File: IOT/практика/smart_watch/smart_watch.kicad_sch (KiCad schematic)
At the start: 30 parts, among them J1 Conn_01x02_Pin, J2 USB_C_Receptacle_USB2.0_16P, SW3 SW_Push, U3 KXTJ3-1057, U4 MAX30102, U5 TPS61230DRC, U6 BQ24090DGQ, U7 ESP32-WROOM-32, U8 LC709203FQH-01TWG

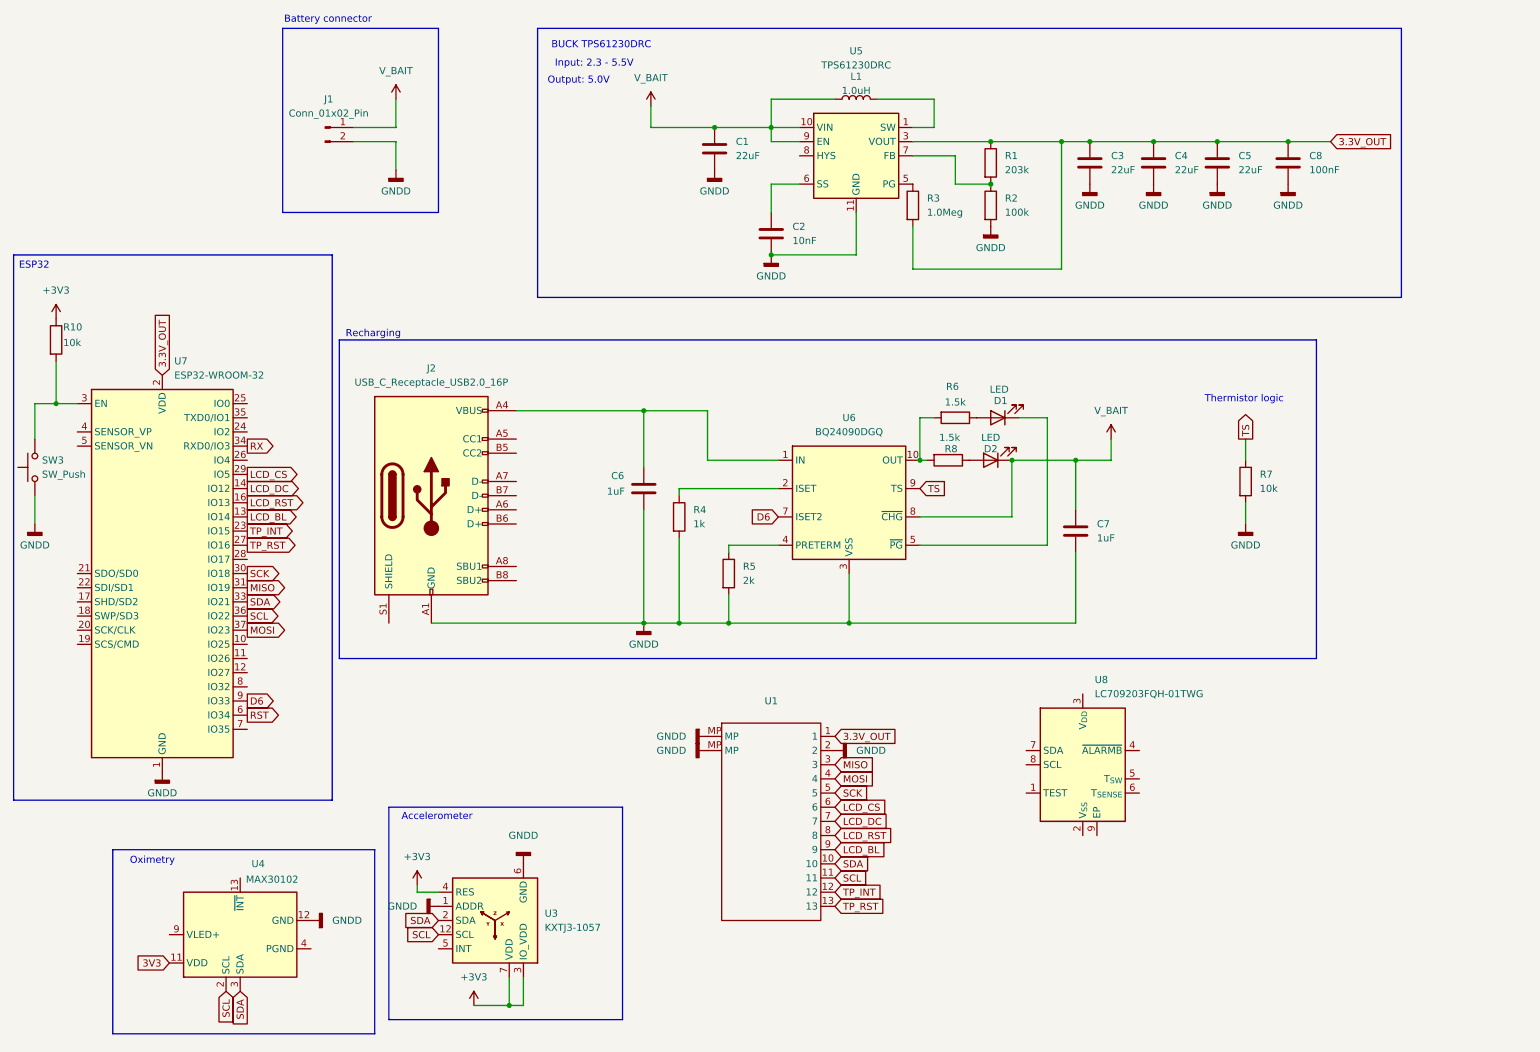
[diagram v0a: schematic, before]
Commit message: updating smart watch
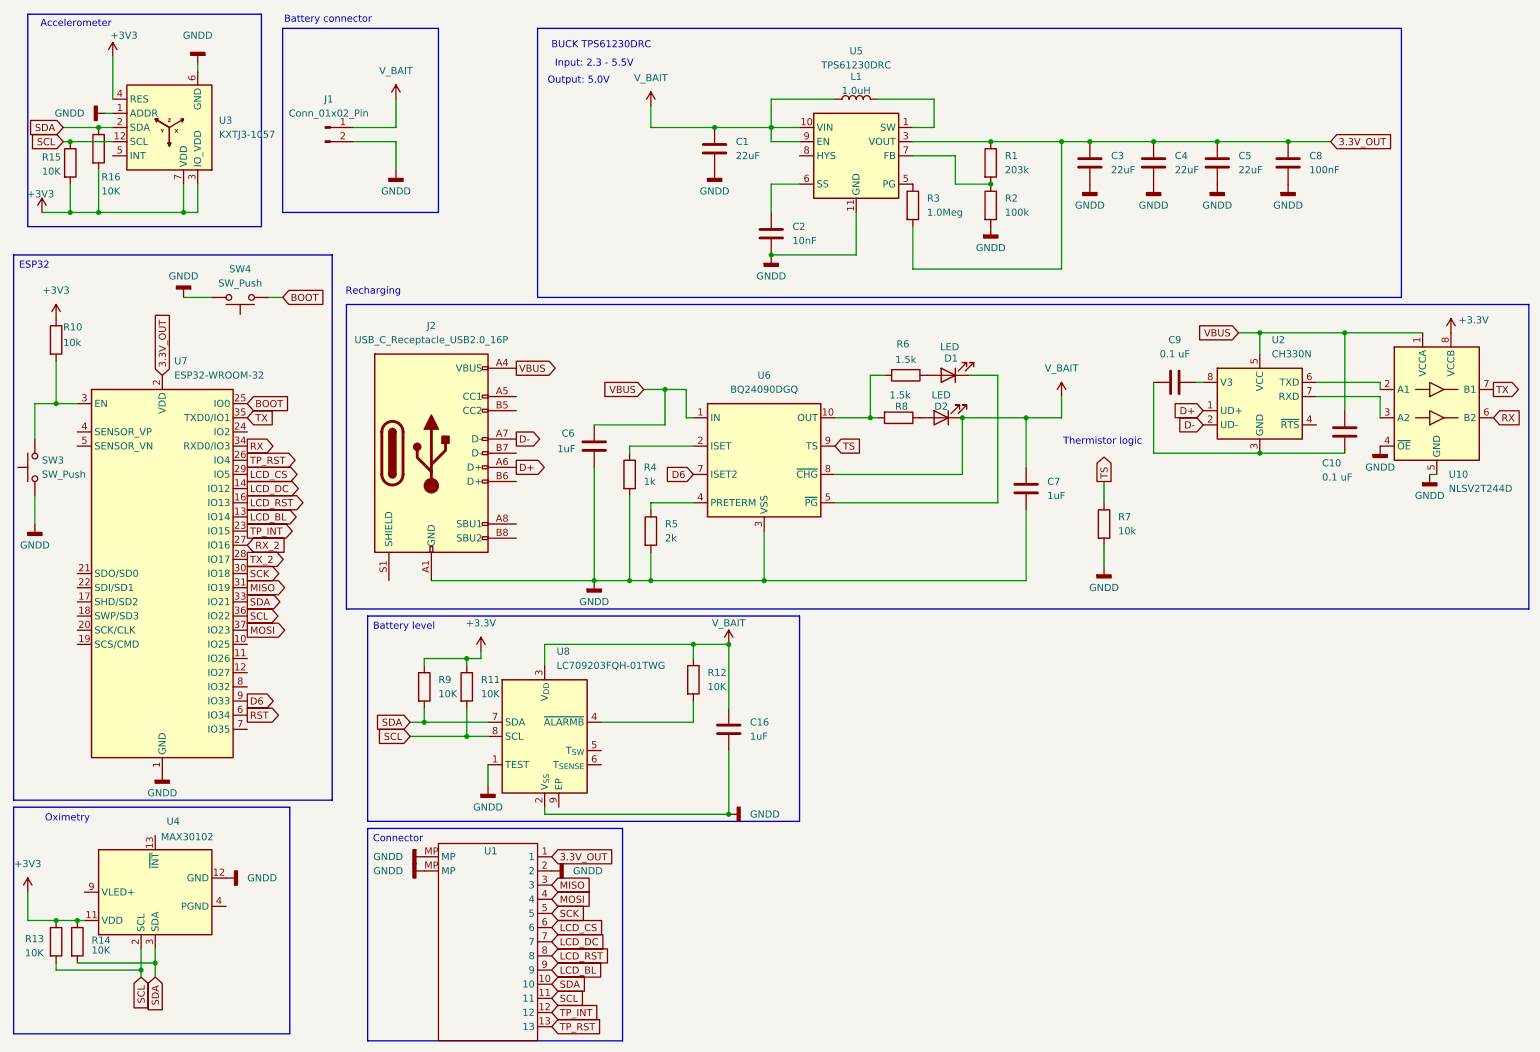
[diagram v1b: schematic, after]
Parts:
- added C10, C9: 0.1 uF, Capacitor_SMD:C_0603_1608Metric, symbol Device:C
- added C16: 1uF, Capacitor_SMD:C_0603_1608Metric, symbol Device:C
- added R11, R12, R13, R14, R15, R16, R9: 10K, Resistor_SMD:R_0603_1608Metric, symbol Device:R
- added SW4: SW_Push, Button_Switch_SMD:SW_Push_1P1T_NO_CK_KMR2, symbol Switch:SW_Push
- added U10: NLSV2T244D, Package_SO:SOIC-8_3.9x4.9mm_P1.27mm, symbol Logic_LevelTranslator:NLSV2T244D
- added U2: CH330N, Package_SO:SOIC-8_3.9x4.9mm_P1.27mm, symbol Interface_USB:CH330N
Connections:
- net 3V3 is gone; now on net +3V3: U4.11 (VDD)
- net +3V3: now also R13.1, R14.1, R15.2, R16.2
- net GNDD: now also U8.1 (TEST), U8.2 (V_{SS}), C16.2, SW4.2, U10.4 (~{OE}), U10.5 (GND)
- net RX: now also U10.6 (B2)
- net SCL: now also U8.8 (SCL), R11.2, R13.2, R15.1
- net SDA: now also U8.7 (SDA), R14.2, R16.1, R9.2
- net TP_RST: now also U7.26 (IO4); no longer U7.27 (IO16)
- net V_BAIT: now also U8.3 (V_{DD}), C16.1, R12.1
- net VBUS: now reaches C6.1, J2.A4 (VBUS), J2.A9 (VBUS), J2.B4 (VBUS), J2.B9 (VBUS), U6.1 (IN)
- net VBUS: now also C10.1, U10.1 (VCCA), U2.5 (VCC)
- net BOOT: now reaches U7.25 (IO0)
- net BOOT: now also SW4.1
- net TX_2: now reaches U7.28 (IO17)
- net TX: now reaches U7.35 (TXD0/IO1)
- net TX: now also U10.7 (B1)
- net at U8.4 (~{ALARMB}): now also R12.2
- net D+: now reaches J2.A6 (D+)
- net D+: now also U2.1 (UD+)
- net D-: now reaches J2.A7 (D-)
- net D-: now also U2.2 (UD-)
- new net: U10.2 (A1), U2.6 (TXD)
- new net: U10.3 (A2), U2.7 (RXD)
- new net: C10.2, C9.1, U2.3 (GND)
- new net: C9.2, U2.8 (V3)
- new net +3.3V: R11.1, R9.1, U10.8 (VCCB)
- new net RX_2: U7.27 (IO16)
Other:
- moved on the sheet: C6, C7, D1, D2, J2, R4, R5, R6, R7, R8, U1, U3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

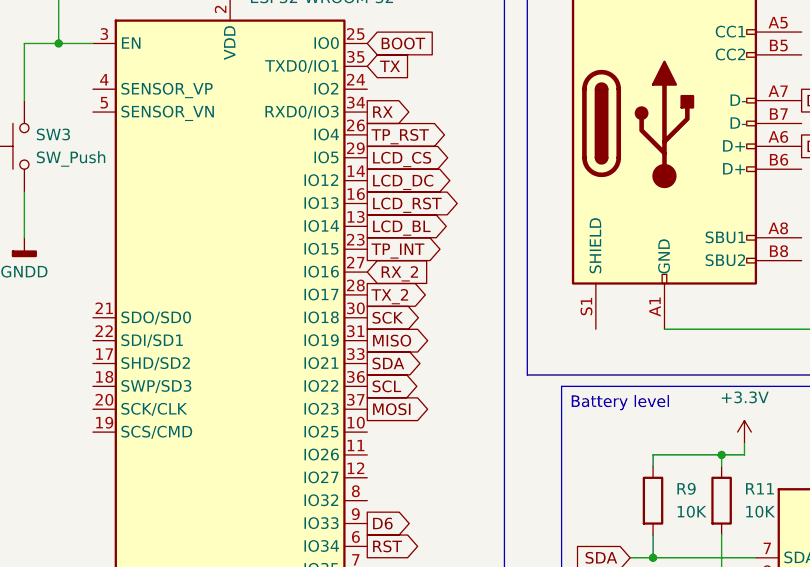
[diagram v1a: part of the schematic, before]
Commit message: updating smart watch
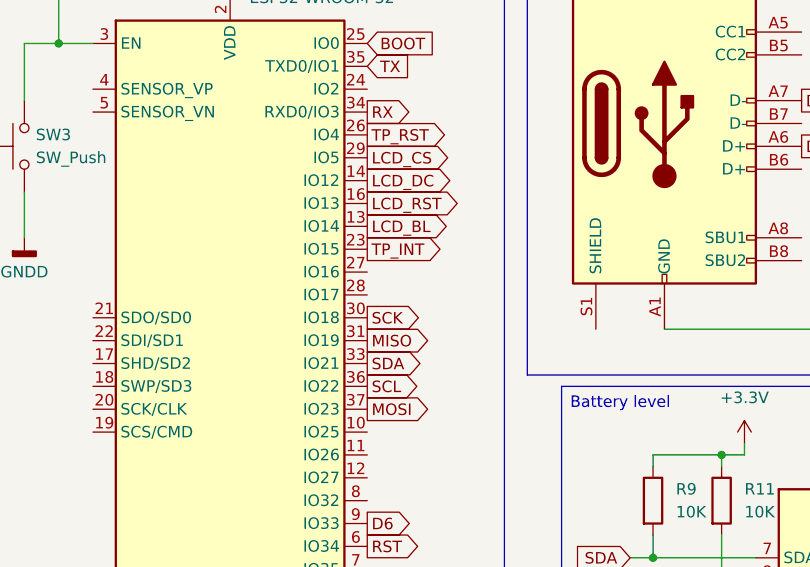
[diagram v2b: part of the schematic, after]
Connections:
- net RX_2: no longer names the net of U7.27 (IO16)
- net TX_2: no longer names the net of U7.28 (IO17)
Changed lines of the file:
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@@
-		)
-	)
-	(global_label "TX_2"
-		(shape output)
-		(at 54.61 111.76 0)
-		(fields_autoplaced yes)
-		(effects
-			(font
-				(size 1.27 1.27)
-			)
-			(justify left)
-		)
-		(property "Intersheetrefs" "${INTERSHEET_REFS}"
-			(at 61.9494 111.76 0)
-			(effects
-				(font
-					(size 1.27 1.27)
-				)
-				(justify left)
-				(hide yes)
-			)
 		)
 	)
@@
 			(effects
 				(font
-					(size 1.27 1.27)
-				)
-				(justify left)
-				(hide yes)
-			)
-		)
-	)
-	(global_label "RX_2"
-		(shape input)
-		(at 54.61 109.22 0)
-		(fields_autoplaced yes)
-		(effects
-			(font
-				(size 1.27 1.27)
-			)
-			(justify left)
-		)
-		(property "Intersheetrefs" "${INTERSHEET_REFS}"
-			(at 62.2518 109.22 0)
-			(effects
-				(font
